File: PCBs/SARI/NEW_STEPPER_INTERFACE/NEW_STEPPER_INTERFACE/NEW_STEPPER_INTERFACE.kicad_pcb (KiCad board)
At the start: 2 copper layers, 97.9 x 53.3 mm, 24 parts, among them J1 TO SARI, J11 STEPPER IN 12-20VDC, J2 MICRO STEP, J3 FROM ARDUINO, J5 ROLL STEPPER, J6 HOZ STEPPER, J7 VERT STEPPER, J8 WTR STEPPER, J9 SLIP STEPPER

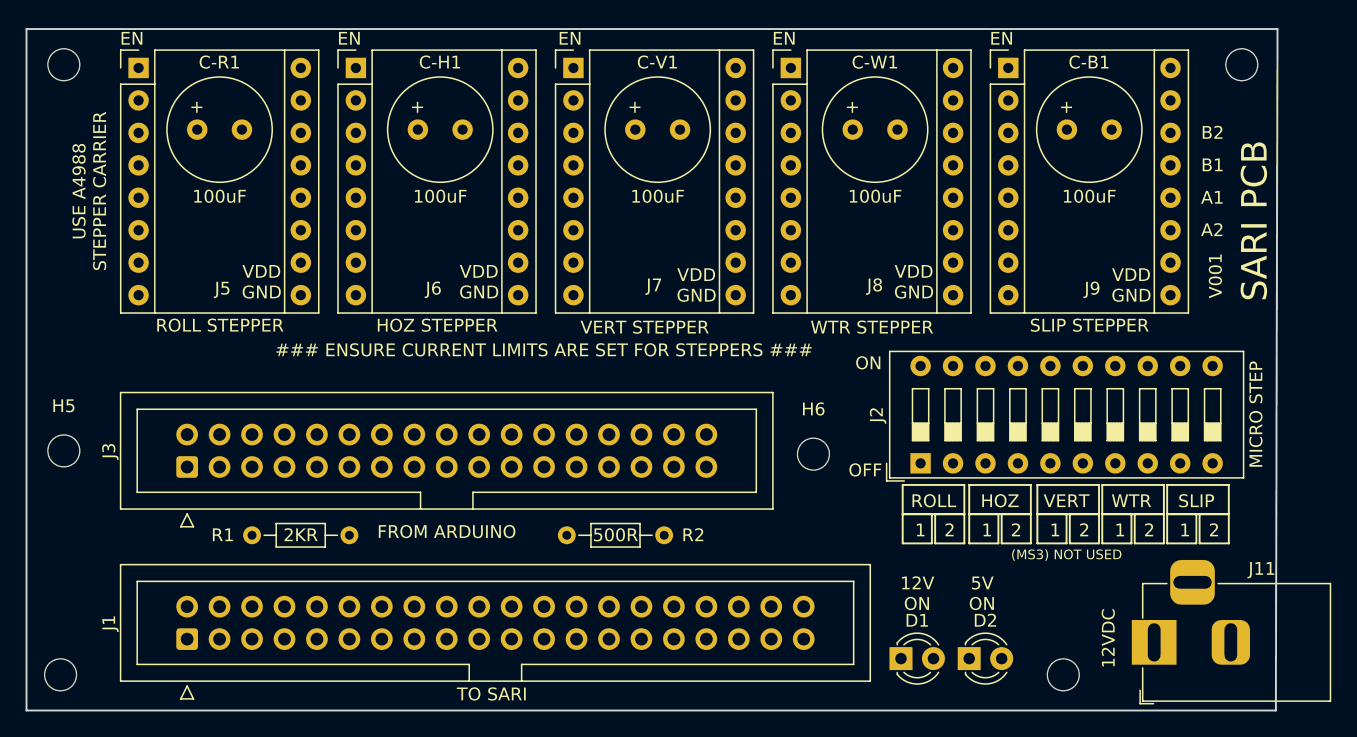
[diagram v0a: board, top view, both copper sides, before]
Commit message: PCB
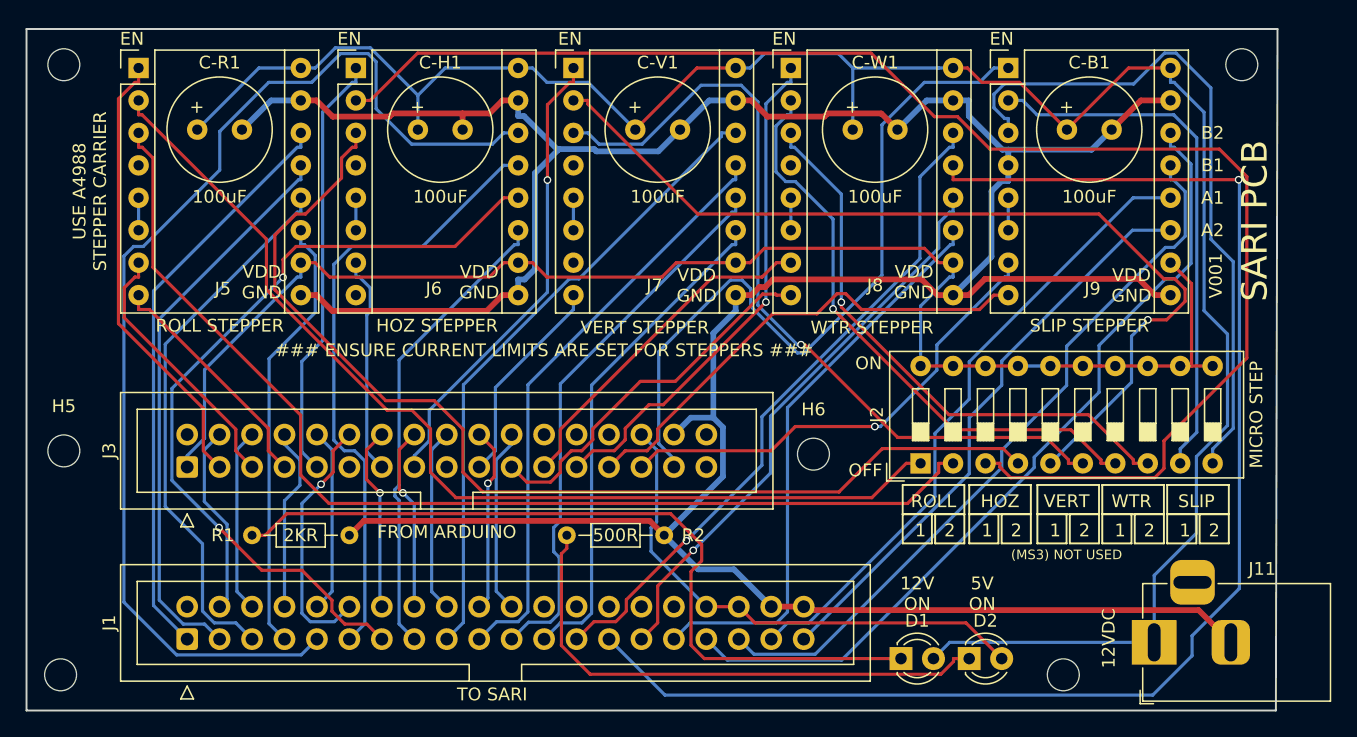
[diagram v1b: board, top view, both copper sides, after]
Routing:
- net GNDD: track 0.00 -> 265.4 mm
- net /BALL_STEP_V+: track 0.00 -> 164.8 mm
- net /HOZ_MS1: track 0.00 -> 115.7 mm
- net /VDD: track 0.00 -> 114.6 mm
- net /WL_1A: track 0.00 -> 111.0 mm, vias 0 -> 1
- net /HOZ_1B: track 0.00 -> 89.1 mm
- net /ROLL_MS2: track 0.00 -> 85.9 mm
- net /HOZ_MS2: track 0.00 -> 84.1 mm
- net /ROLL_MS1: track 0.00 -> 80.2 mm
- net /VER_MS1: track 0.00 -> 73.0 mm, vias 0 -> 1
- net /BALL_1B: track 0.00 -> 65.1 mm
- net /VER_MS2: track 0.00 -> 63.9 mm, vias 0 -> 1
- net /HOZ_2A: track 0.00 -> 63.4 mm, vias 0 -> 2
- net Net-(D1-Pad1): track 0.00 -> 62.0 mm
- net /BALL_EN: track 0.00 -> 58.5 mm
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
